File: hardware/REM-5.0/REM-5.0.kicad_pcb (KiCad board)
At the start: 2 copper layers, 98.4 x 44.5 mm, 35 parts, among them J1 PinHeader_2.54mm 02x04 Horizo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, J2 PinHeader_2.54mm 02x05 Horizo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, Q1 IRLB3034PbF, Q2 BCX56, Q3 BCX53, U2 74LVC1G14

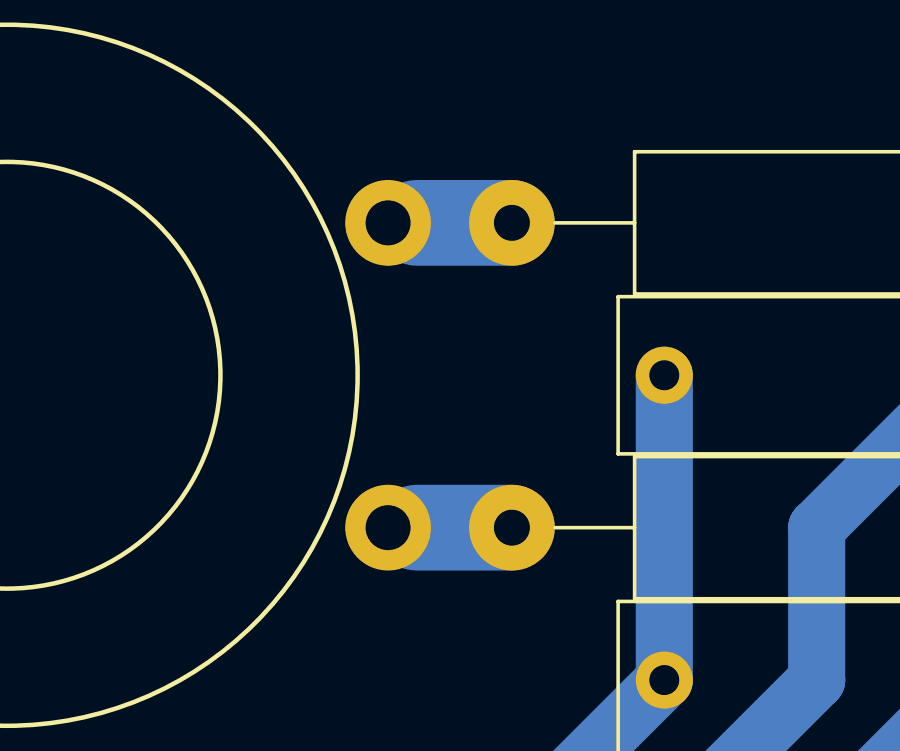
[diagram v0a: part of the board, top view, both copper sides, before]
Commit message: new file:   firmware/ESP32-S3 PWM/.cache/clangd/index/Alignment.hpp.726B1D6F8AC0E5FC.idx 	new file:   firmware/ESP32-S3 PWM/.cache/clangd/index/ArduinoJson.h.11C8086DC5DC1D39.idx 	new file:   firmware/ESP32-S3 PWM/.cache/clangd/index/ArduinoJson.hpp.7FAD813322DCFBBA.idx 	new file:   firmware/ESP32-S3 PWM/.cache/clangd/index/ArduinoStreamReader.hpp.6A6C10A39AA283AA.idx 	new file:   firmware/ESP32-S3 PWM/.cache/clangd/index/ArduinoStringReader.hpp.4194E32BF9D83CDF.idx 	new file:   firmware/ESP32-S3 PWM/.cache/clangd/index/ArduinoStringWriter.hpp.B2A9673B221215CD.idx 	new file:   firmware/ESP32-S3 PWM/.cache/clangd/index/BasicJsonDocument.hpp.FF9A72F18774339B.idx 	new file:   firmware/ESP32-S3 PWM/.cache/clangd/index/CollectionData.hpp.D0A6E066F6D81A3D.idx 	new file:   firmware/ESP32-S3 PWM/.cache/clangd/index/CollectionImpl.hpp.9A8E7E970CC61A36.idx 	new file:   firmware/ESP32-S3 PWM/.cache/clangd/index/Configuration.hpp.709A1F7F02EFA908.idx 	new file:   firmware/ESP32-S3 PWM/.cache/clangd/index/Converter.hpp.2991290B38DAAF2D.idx 	new file:   firmware/ESP32-S3 PWM/.cache/clangd/index/ConverterImpl.hpp.2B62C8A86CE75E37.idx 	new file:   firmware/ESP32-S3 PWM/.cache/clangd/index/CountingDecorator.hpp.4110D54BC05F9B43.idx 	new file:   firmware/ESP32-S3 PWM/.cache/clangd/index/DeserializationError.hpp.EFFDB4C051A5880A.idx 	new file:   firmware/ESP32-S3 PWM/.cache/clangd/index/DeserializationOptions.hpp.D0990CE9A84F0543.idx 	new file:   firmware/ESP32-S3 PWM/.cache/clangd/index/DummyWriter.hpp.436C5532B841A3A4.idx 	new file:   firmware/ESP32-S3 PWM/.cache/clangd/index/DynamicJsonDocument.hpp.DEEADBD70694B4BE.idx 	new file:   firmware/ESP32-S3 PWM/.cache/clangd/index/ElementProxy.hpp.209B2FA01DA5C38D.idx 	new file:   firmware/ESP32-S3 PWM/.cache/clangd/index/EscapeSequence.hpp.0E535D59050D1B63.idx 	new file:   firmware/ESP32-S3 PWM/.cache/clangd/index/Filter.hpp.2866D748202E02C1.idx 	new file:   firmware/ESP32-S3 PWM/.cache/clangd/index/FlashReader.hpp.A4CB3621CFAD50BE.idx 	n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
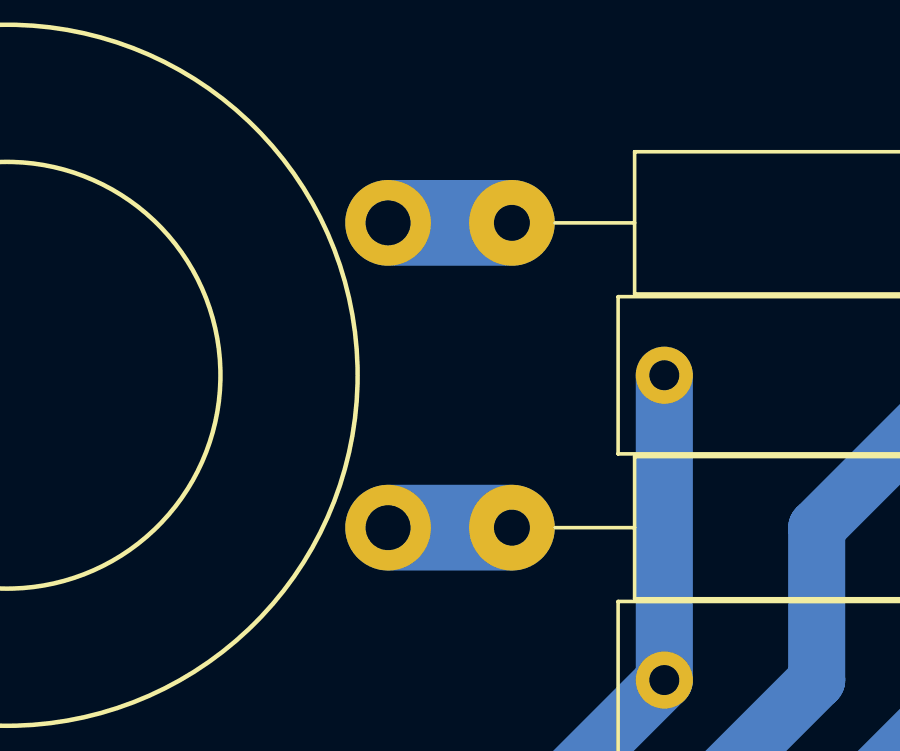
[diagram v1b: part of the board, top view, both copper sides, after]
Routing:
- net Net-(L1-Pad4): track 3.17 -> 4.13 mm
- net Net-(L1-Pad3): track 3.17 -> 4.13 mm
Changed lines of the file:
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@@
 		)
 		(property "Value" "0.01µF 1000"
-			(at 4.999999 3.75 360)
+			(at 4.999999 3.75 0)
 			(layer "F.Fab")
 			(effects
@@
 		)
 		(fp_text user "${REFERENCE}"
-			(at 5 0 360)
+			(at 5 0 0)
 			(layer "F.Fab")
 			(effects
@@
 	)
 	(footprint "Connector_PinHeader_2.54mm:PinHeader_1x03_P5.08mm_Horizontal_2"
+		(locked yes)
 		(layer "F.Cu")
 		(at 180.0225 104.29875 -90)
@@
 		(tags "Resistor Axial_DIN0414 series Axial Horizontal pin pitch 20.32mm 2W length 11.9mm diameter 4.5mm")
 		(property "Reference" "R9"
-			(at 0 -3.37 360)
+			(at 0 -3.37 0)
 			(layer "F.SilkS")
 			(hide yes)
@@
 		)
 		(property "Value" "33Ω 2W"
-			(at 0 3.37 360)
+			(at 0 3.37 0)
 			(layer "F.Fab")
 			(effects
@@
 		)
 		(fp_text user "${REFERENCE}"
-			(at 0 0 360)
+			(at 0 0 0)
 			(layer "F.Fab")
 			(effects
@@
 		)
 		(property "Value" "0.01µF 1000"
-			(at 4.999999 3.75 360)
+			(at 4.999999 3.75 0)
 			(layer "F.Fab")
 			(effects
@@
 		)
 		(fp_text user "${REFERENCE}"
-			(at 5 0 360)
+			(at 5 0 0)
 			(layer "F.Fab")
 			(effects
@@
 		(tags "capacitor tantalum")
 		(property "Reference" "C7"
-			(at 0 -3.1 360)
+			(at 0 -3.1 0)
 			(layer "F.SilkS")
 			(hide yes)
@@
 		)
 		(property "Value" "470uF 16V"
-			(at 0 3.1 360)
+			(at 0 3.1 0)
 			(layer "F.Fab")
 			(effects
@@
 		)
 		(fp_text user "${REFERENCE}"
-			(at 0 0 360)
+			(at 0 0 0)
 			(layer "F.Fab")
 			(effects
@@
 	(segment
 		(start 169.2275 79.375001)
-		(end 166.0525 79.375001)
+		(end 165.1 79.375001)
 		(width 2.8575)
 		(layer "B.Cu")
@@
 	(segment
 		(start 169.2275 89.535001)
-		(end 166.0525 89.535001)
+		(end 165.1 89.535001)
 		(width 2.8575)
 		(layer "B.Cu")

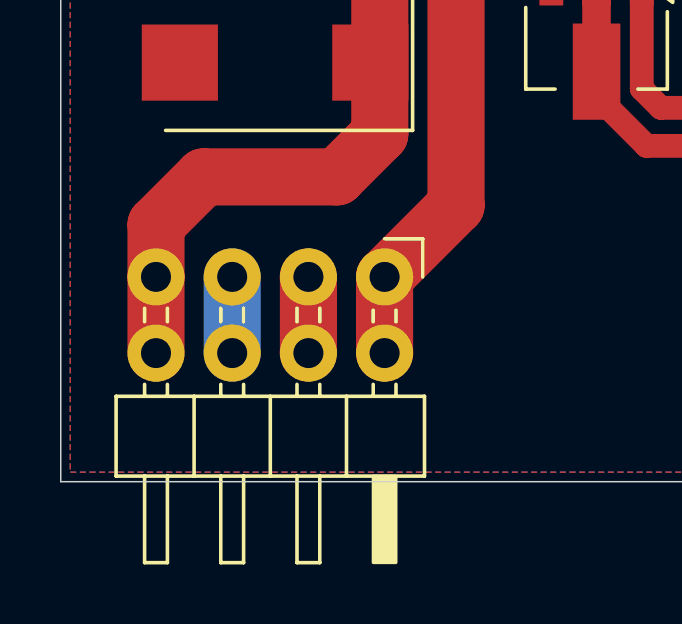
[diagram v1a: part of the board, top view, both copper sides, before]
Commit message: modified:   firmware/ESU_V1/include/data_manager.h 	modified:   firmware/ESU_V1/include/hardware_control.h 	modified:   firmware/ESU_V1/src/hardware_control.cpp 	modified:   firmware/ESU_V1/src/main.cpp 	modified:   hardware/CTL-6.1/CTL-6.1.kicad_pcb 	modified:   hardware/CTL-6.1/CTL-6.1.kicad_prl 	modified:   hardware/CTL-6.1/CTL-6.1.kicad_pro 	modified:   hardware/INA-3/INA-3.kicad_pcb 	modified:   hardware/INA-3/INA-3.kicad_prl 	modified:   hardware/INA-3/INA-3.kicad_pro 	modified:   hardware/INA-3/INA-3.kicad_sch 	renamed:    hardware/INA-3/fabrication-outputs/INA-3-TRACE.dxf -> hardware/INA-3/fabrication-outputs/EDGE.dxf 	deleted:    hardware/INA-3/fabrication-outputs/INA-3-Edge_Cuts.dxf 	modified:   hardware/INA-3/fabrication-outputs/INA-3-F_Cu.dxf 	new file:   hardware/INA-3/fabrication-outputs/INA-3-F_Cu.pdf 	deleted:    hardware/INA-3/fabrication-outputs/INA-3-NPTH-drl_map.dxf 	deleted:    hardware/INA-3/fabrication-outputs/INA-3-PTH-drl_map.dxf 	new file:   hardware/INA-3/fabrication-outputs/TRACE.dxf 	deleted:    hardware/INA-3/fp-info-cache 	new file:   hardware/REM-5.0/.history 	modified:   hardware/REM-5.0/REM-5.0.kicad_pcb 	modified:   hardware/REM-5.0/REM-5.0.kicad_prl 	modified:   hardware/REM-5.0/REM-5.0.kicad_pro
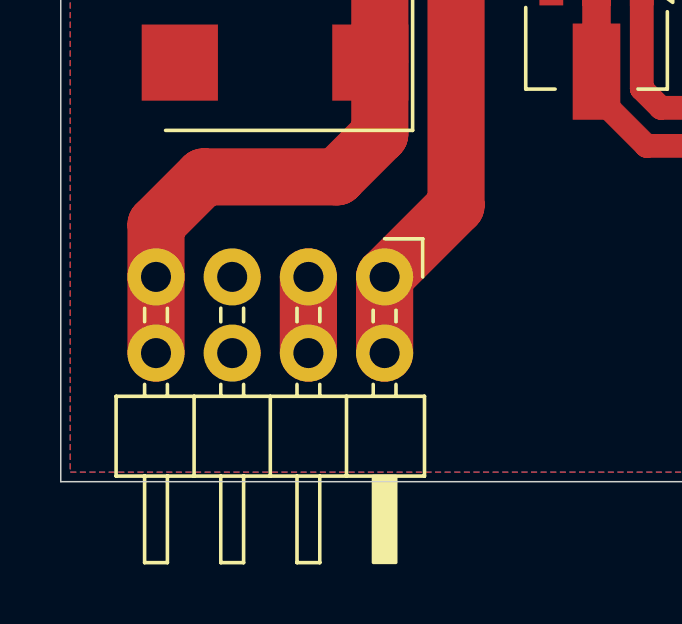
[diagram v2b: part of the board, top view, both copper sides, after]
